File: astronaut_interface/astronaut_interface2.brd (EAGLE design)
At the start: 61.9 x 53.3 mm, 17 parts, among them IC1 PCF8591T, J1 UI, J2 Display, P1 JT9S-19, U1 TACT-12MM, U2 TACT-12MM, U3 TACT-12MM, U4 TACT-12MM

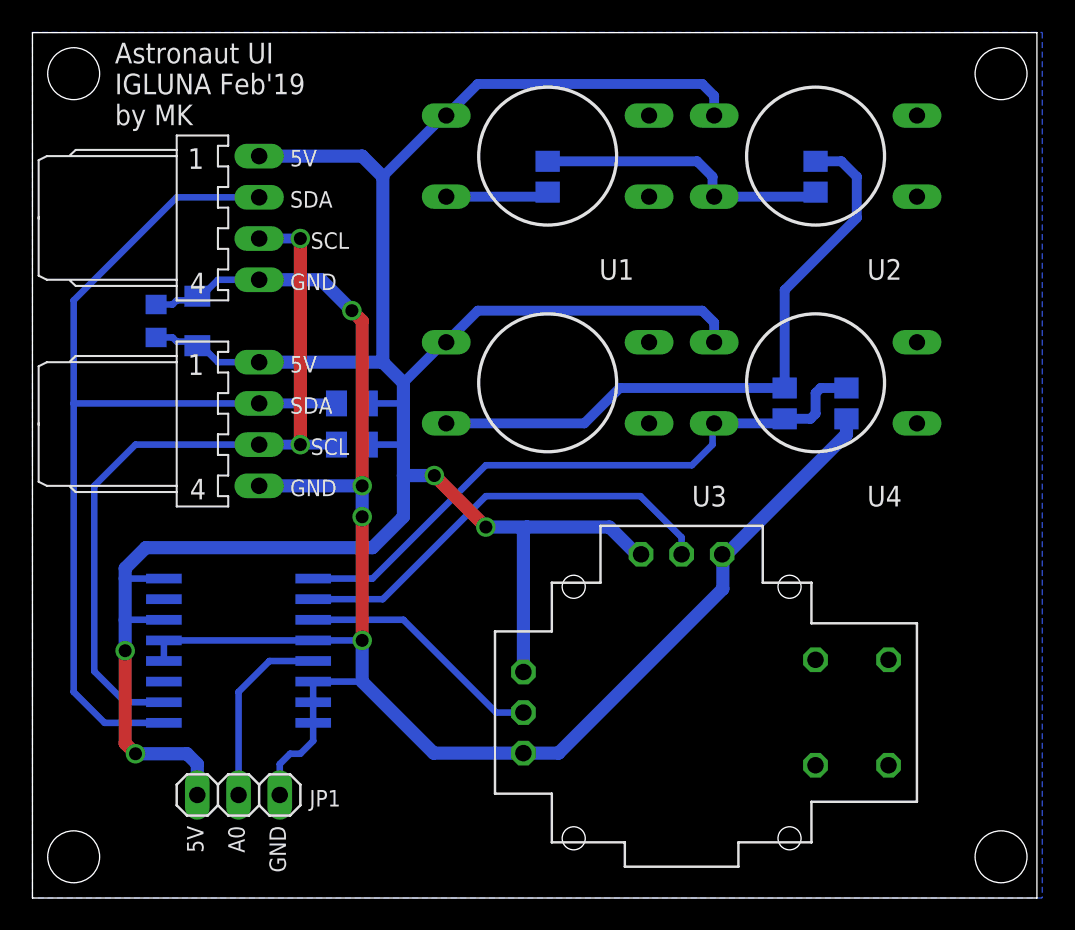
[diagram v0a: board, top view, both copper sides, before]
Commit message: verified, ready to production
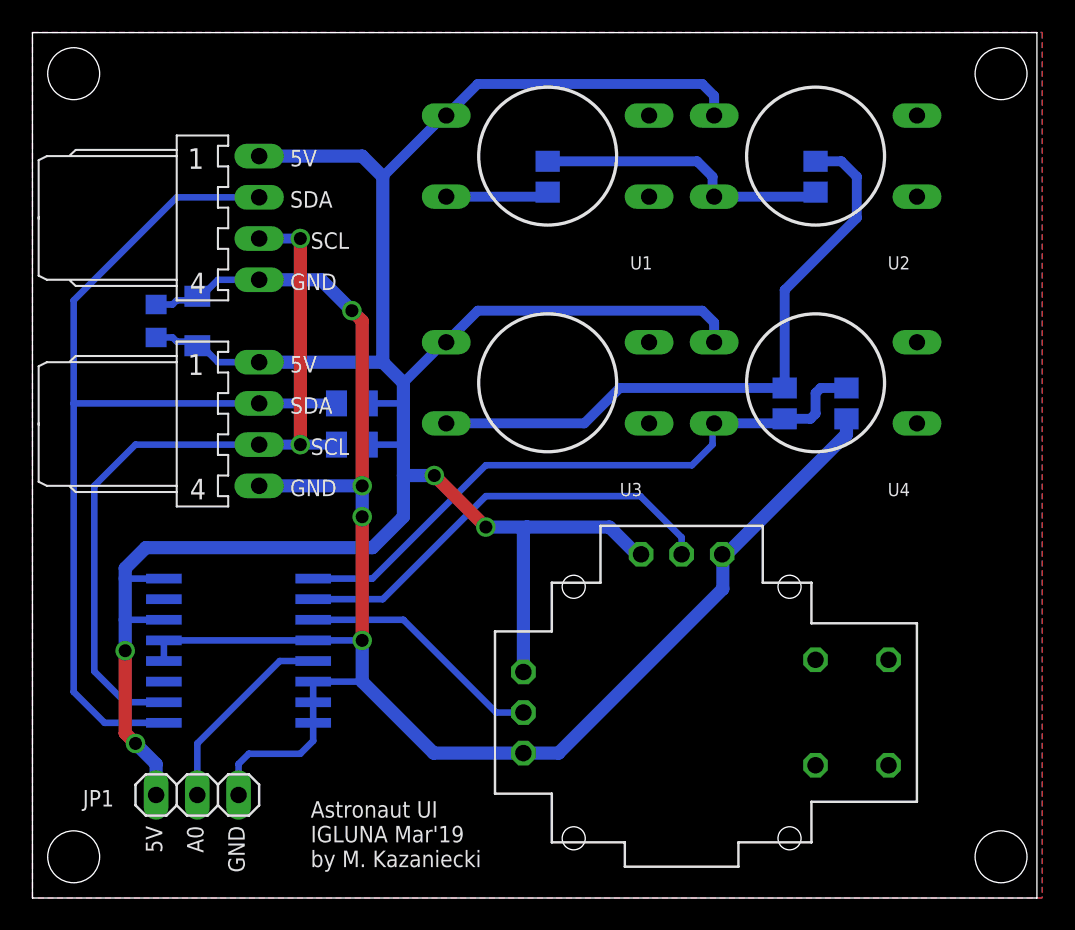
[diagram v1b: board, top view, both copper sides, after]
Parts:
- moved JP1 2.54 mm to (12.7, 6.35)
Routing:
- net +5V: track 162.9 -> 160.0 mm
- net GND: track 109.7 -> 112.3 mm
- net A0: track 11.7 -> 12.4 mm
- added copper zone on layer 1, net GND
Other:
- board text added: "Astronaut UI IGLUNA Mar'19 by M. Kazaniecki"
- board text removed: "Astronaut UI IGLUNA Feb'19 by MK"
- board text removed: "prostokąt to moduł wyświetlacza 4x20 (całe PCB)"

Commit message: final, after another review
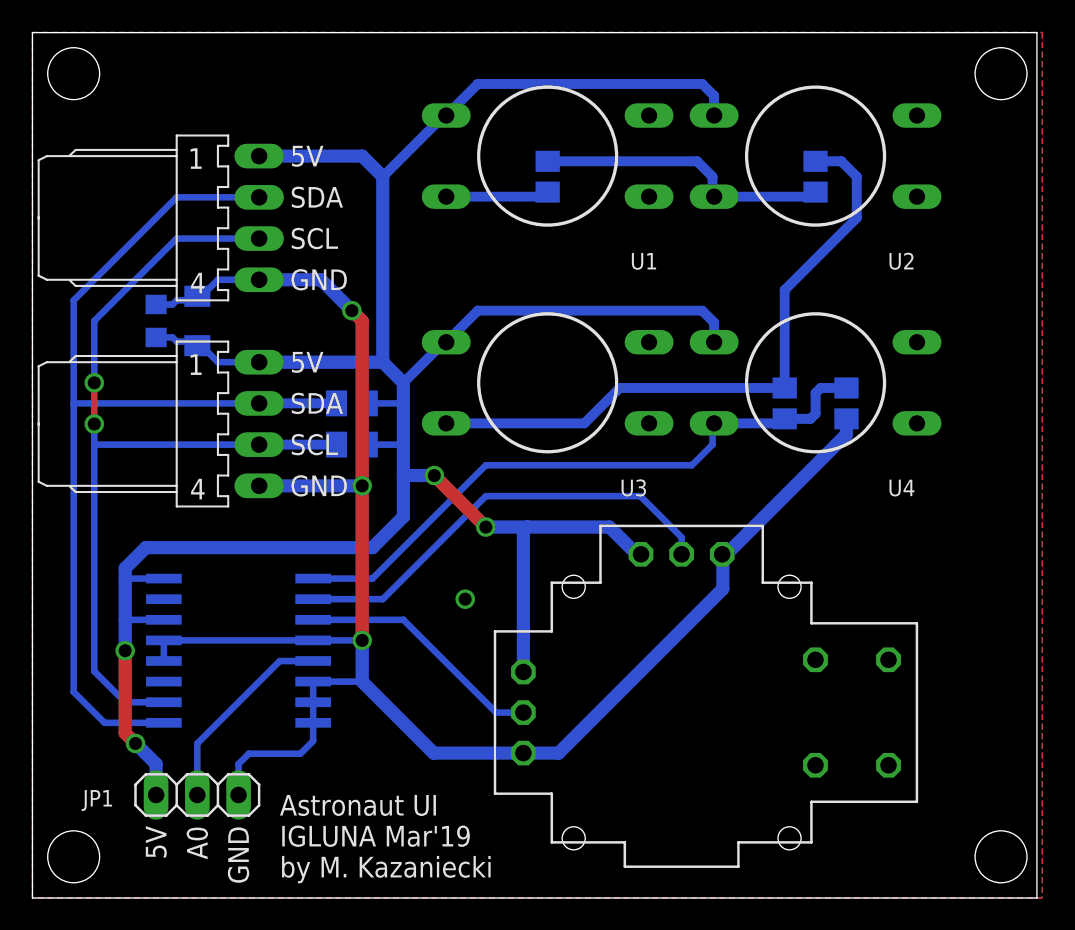
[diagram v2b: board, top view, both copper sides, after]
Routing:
- net I2C_SCL: track 47.7 -> 53.9 mm

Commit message: really final projects, added gerber files
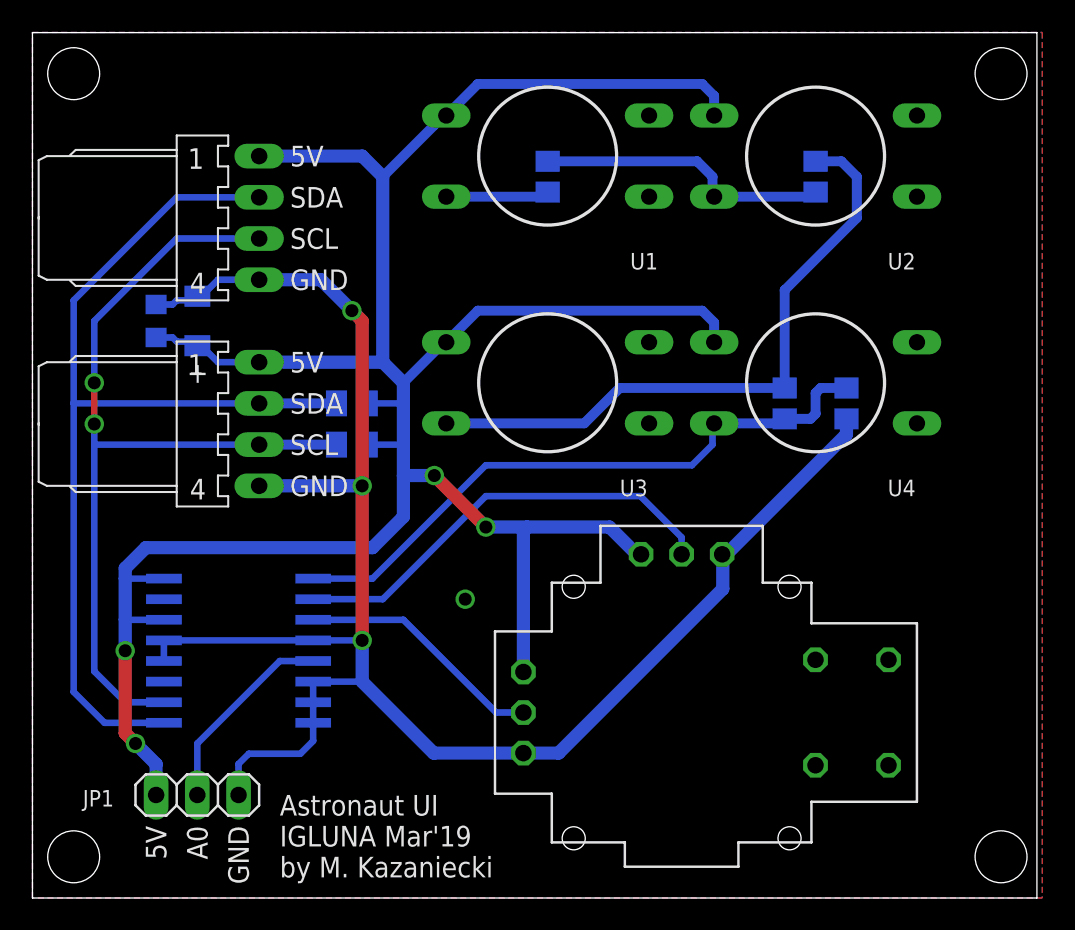
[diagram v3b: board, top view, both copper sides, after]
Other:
- board text added: "+"
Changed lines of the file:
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@@
 <layer number="19" name="Unrouted" color="6" fill="1" visible="yes" active="yes"/>
 <layer number="20" name="Dimension" color="15" fill="1" visible="yes" active="yes"/>
-<layer number="21" name="tPlace" color="7" fill="1" visible="yes" active="yes"/>
-<layer number="22" name="bPlace" color="7" fill="1" visible="yes" active="yes"/>
+<layer number="21" name="tPlace" color="7" fill="1" visible="no" active="yes"/>
+<layer number="22" name="bPlace" color="7" fill="1" visible="no" active="yes"/>
 <layer number="23" name="tOrigins" color="15" fill="1" visible="yes" active="yes"/>
 <layer number="24" name="bOrigins" color="15" fill="1" visible="yes" active="yes"/>
@@
 <layer number="27" name="tValues" color="7" fill="1" visible="yes" active="yes"/>
 <layer number="28" name="bValues" color="7" fill="1" visible="yes" active="yes"/>
-<layer number="29" name="tStop" color="7" fill="3" visible="no" active="yes"/>
-<layer number="30" name="bStop" color="7" fill="6" visible="no" active="yes"/>
-<layer number="31" name="tCream" color="7" fill="4" visible="no" active="yes"/>
-<layer number="32" name="bCream" color="7" fill="5" visible="no" active="yes"/>
-<layer number="33" name="tFinish" color="6" fill="3" visible="no" active="yes"/>
-<layer number="34" name="bFinish" color="6" fill="6" visible="no" active="yes"/>
-<layer number="35" name="tGlue" color="7" fill="4" visible="no" active="yes"/>
-<layer number="36" name="bGlue" color="7" fill="5" visible="no" active="yes"/>
-<layer number="37" name="tTest" color="7" fill="1" visible="no" active="yes"/>
-<layer number="38" name="bTest" color="7" fill="1" visible="no" active="yes"/>
+<layer number="29" name="tStop" color="7" fill="3" visible="yes" active="yes"/>
+<layer number="30" name="bStop" color="7" fill="6" visible="yes" active="yes"/>
+<layer number="31" name="tCream" color="7" fill="4" visible="yes" active="yes"/>
+<layer number="32" name="bCream" color="7" fill="5" visible="yes" active="yes"/>
+<layer number="33" name="tFinish" color="6" fill="3" visible="yes" active="yes"/>
+<layer number="34" name="bFinish" color="6" fill="6" visible="yes" active="yes"/>
+<layer number="35" name="tGlue" color="7" fill="4" visible="yes" active="yes"/>
+<layer number="36" name="bGlue" color="7" fill="5" visible="yes" active="yes"/>
+<layer number="37" name="tTest" color="7" fill="1" visible="yes" active="yes"/>
+<layer number="38" name="bTest" color="7" fill="1" visible="yes" active="yes"/>
 <layer number="39" name="tKeepout" color="4" fill="11" visible="yes" active="yes"/>
 <layer number="40" name="bKeepout" color="1" fill="11" visible="yes" active="yes"/>
@@
 <layer number="42" name="bRestrict" color="1" fill="10" visible="yes" active="yes"/>
 <layer number="43" name="vRestrict" color="2" fill="10" visible="yes" active="yes"/>
-<layer number="44" name="Drills" color="7" fill="1" visible="no" active="yes"/>
+<layer number="44" name="Drills" color="7" fill="1" visible="yes" active="yes"/>
 <layer number="45" name="Holes" color="7" fill="1" visible="yes" active="yes"/>
-<layer number="46" name="Milling" color="3" fill="1" visible="no" active="yes"/>
-<layer number="47" name="Measures" color="7" fill="1" visible="no" active="yes"/>
+<layer number="46" name="Milling" color="3" fill="1" visible="yes" active="yes"/>
+<layer number="47" name="Measures" color="7" fill="1" visible="yes" active="yes"/>
 <layer number="48" name="Document" color="7" fill="1" visible="yes" active="yes"/>
 <layer number="49" name="Reference" color="7" fill="1" visible="yes" active="yes"/>
@@
 <layer number="112" name="tSilk" color="7" fill="1" visible="yes" active="yes"/>
 <layer number="113" name="IDFDebug" color="4" fill="1" visible="yes" active="yes"/>
-<layer number="114" name="Badge_Outline" color="7" fill="1" visible="no" active="yes"/>
-<layer number="115" name="ReferenceISLANDS" color="7" fill="1" visible="no" active="yes"/>
+<layer number="114" name="Badge_Outline" color="7" fill="1" visible="yes" active="yes"/>
+<layer number="115" name="ReferenceISLANDS" color="7" fill="1" visible="yes" active="yes"/>
 <layer number="116" name="Patch_BOT" color="9" fill="4" visible="yes" active="yes"/>
-<layer number="118" name="Rect_Pads" color="7" fill="1" visible="no" active="yes"/>
+<layer number="118" name="Rect_Pads" color="7" fill="1" visible="yes" active="yes"/>
 <layer number="121" name="_tsilk" color="7" fill="1" visible="yes" active="yes"/>
 <layer number="122" name="_bsilk" color="7" fill="1" visible="yes" active="yes"/>
@@
 <text x="14.605" y="4.445" size="1.27" layer="25" font="vector" ratio="15" rot="R270">GND</text>
 <text x="12.065" y="4.445" size="1.27" layer="25" font="vector" ratio="15" rot="R270">A0</text>
+<text x="12.065" y="31.75" size="1.27" layer="25" font="vector" ratio="15">+</text>
 </plain>
 <attributes>
@@
 </class>
 </classes>
-<designrules name="default *">
+<designrules name="jlcpcb_rules">
 <description language="de">&lt;b&gt;EAGLE Design Rules&lt;/b&gt;
 &lt;p&gt;
@@
 <param name="mtCopper" value="0.035mm 0.035mm 0.035mm 0.035mm 0.035mm 0.035mm 0.035mm 0.035mm 0.035mm 0.035mm 0.035mm 0.035mm 0.035mm 0.035mm 0.035mm 0.035mm"/>
 <param name="mtIsolate" value="1.5mm 0.15mm 0.2mm 0.15mm 0.2mm 0.15mm 0.2mm 0.15mm 0.2mm 0.15mm 0.2mm 0.15mm 0.2mm 0.15mm 0.2mm"/>
-<param name="mdWireWire" value="12mil"/>
-<param name="mdWirePad" value="12mil"/>
-<param name="mdWireVia" value="12mil"/>
-<param name="mdPadPad" value="10mil"/>
-<param name="mdPadVia" value="12mil"/>
-<param name="mdViaVia" value="12mil"/>
-<param name="mdSmdPad" value="10mil"/>
-<param name="mdSmdVia" value="10mil"/>
-<param name="mdSmdSmd" value="10mil"/>
-<param name="mdViaViaSameLayer" value="8mil"/>
+<param name="mdWireWire" value="5mil"/>
+<param name="mdWirePad" value="5mil"/>
+<param name="mdWireVia" value="5mil"/>
+<param name="mdPadPad" value="5mil"/>
+<param name="mdPadVia" value="5mil"/>
+<param name="mdViaVia" value="5mil"/>
+<param name="mdSmdPad" value="5mil"/>
+<param name="mdSmdVia" value="5mil"/>
+<param name="mdSmdSmd" value="5mil"/>
+<param name="mdViaViaSameLayer" value="6mil"/>
 <param name="mnLayersViaInSmd" value="2"/>
-<param name="mdCopperDimension" value="20mil"/>
+<param name="mdCopperDimension" value="0.2mm"/>
 <param name="mdDrill" value="12mil"/>
 <param name="mdSmdStop" value="0mil"/>
-<param name="msWidth" value="12mil"/>
-<param name="msDrill" value="24mil"/>
+<param name="msWidth" value="5mil"/>
+<param name="msDrill" value="0.2mm"/>
 <param name="msMicroVia" value="9.99mm"/>
 <param name="msBlindViaRatio" value="0.5"/>
@@
 <param name="rvMicroViaOuter" value="0.25"/>
 <param name="rvMicroViaInner" value="0.25"/>
-<param name="rlMinPadTop" value="10mil"/>
+<param name="rlMinPadTop" value="3mil"/>
 <param name="rlMaxPadTop" value="20mil"/>
 <param name="rlMinPadInner" value="10mil"/>
@@
 <param name="rlMinPadBottom" value="10mil"/>
 <param name="rlMaxPadBottom" value="20mil"/>
-<param name="rlMinViaOuter" value="8mil"/>
+<param name="rlMinViaOuter" value="3mil"/>
 <param name="rlMaxViaOuter" value="20mil"/>
 <param name="rlMinViaInner" value="8mil"/>
@@
 <element name="P1" library="jt9s-1p" package="JT9S-1P" value="JT9S-19" x="42.545" y="11.43" smashed="yes"/>
 <element name="R1" library="rcl" package="R0805" value="1k" x="34.29" y="44.45" smashed="yes" rot="MR270">
-<attribute name="NAME" x="34.29" y="48.26" size="1.016" layer="26" font="vector" ratio="15" rot="MR270"/>
+<attribute name="NAME" x="35.56" y="43.815" size="1.016" layer="26" font="vector" ratio="15" rot="MR90"/>
 </element>
 <element name="R2" library="rcl" package="R0805" value="1k" x="50.8" y="44.45" smashed="yes" rot="MR270">
-<attribute name="NAME" x="50.8" y="48.26" size="1.016" layer="26" font="vector" ratio="15" rot="MR270"/>
+<attribute name="NAME" x="52.07" y="43.815" size="1.016" layer="26" font="vector" ratio="15" rot="MR90"/>
 </element>
 <element name="R3" library="rcl" package="R0805" value="1k" x="48.895" y="30.48" smashed="yes" rot="MR90">
-<attribute name="NAME" x="49.53" y="34.29" size="1.016" layer="26" font="vector" ratio="15" rot="MR270"/>
+<attribute name="NAME" x="50.165" y="29.845" size="1.016" layer="26" font="vector" ratio="15" rot="MR90"/>
 </element>
 <element name="R4" library="rcl" package="R0805" value="1k" x="52.705" y="30.48" smashed="yes" rot="MR90">
-<attribute name="NAME" x="52.705" y="26.67" size="1.016" layer="26" font="vector" ratio="15" rot="MR90"/>
+<attribute name="NAME" x="53.975" y="29.845" size="1.016" layer="26" font="vector" ratio="15" rot="MR90"/>
 </element>
 <element name="R5" library="resistor" package="M0805" value="470" x="22.225" y="27.94" smashed="yes" rot="MR180">
